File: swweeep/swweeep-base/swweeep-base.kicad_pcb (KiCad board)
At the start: 2 copper layers, 113.3 x 89.7 mm, 3 parts

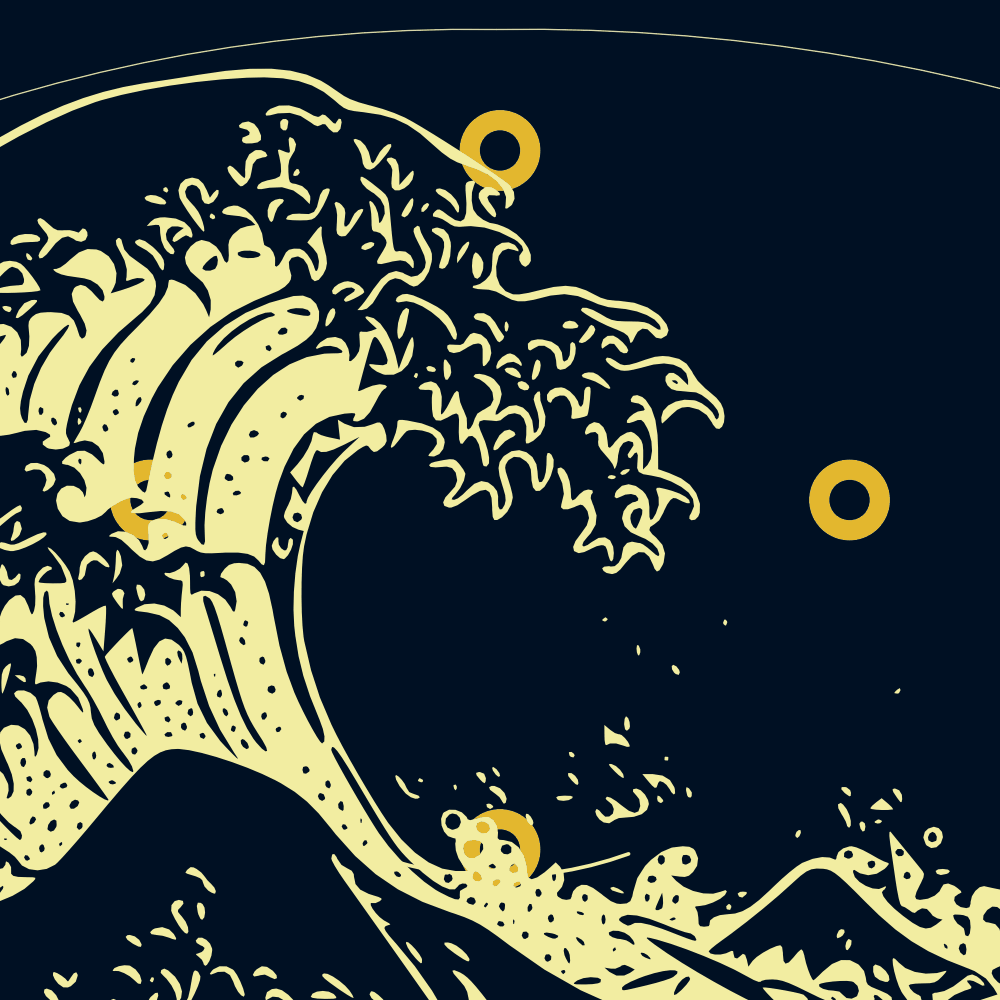
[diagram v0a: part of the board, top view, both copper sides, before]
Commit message: Mess up everything
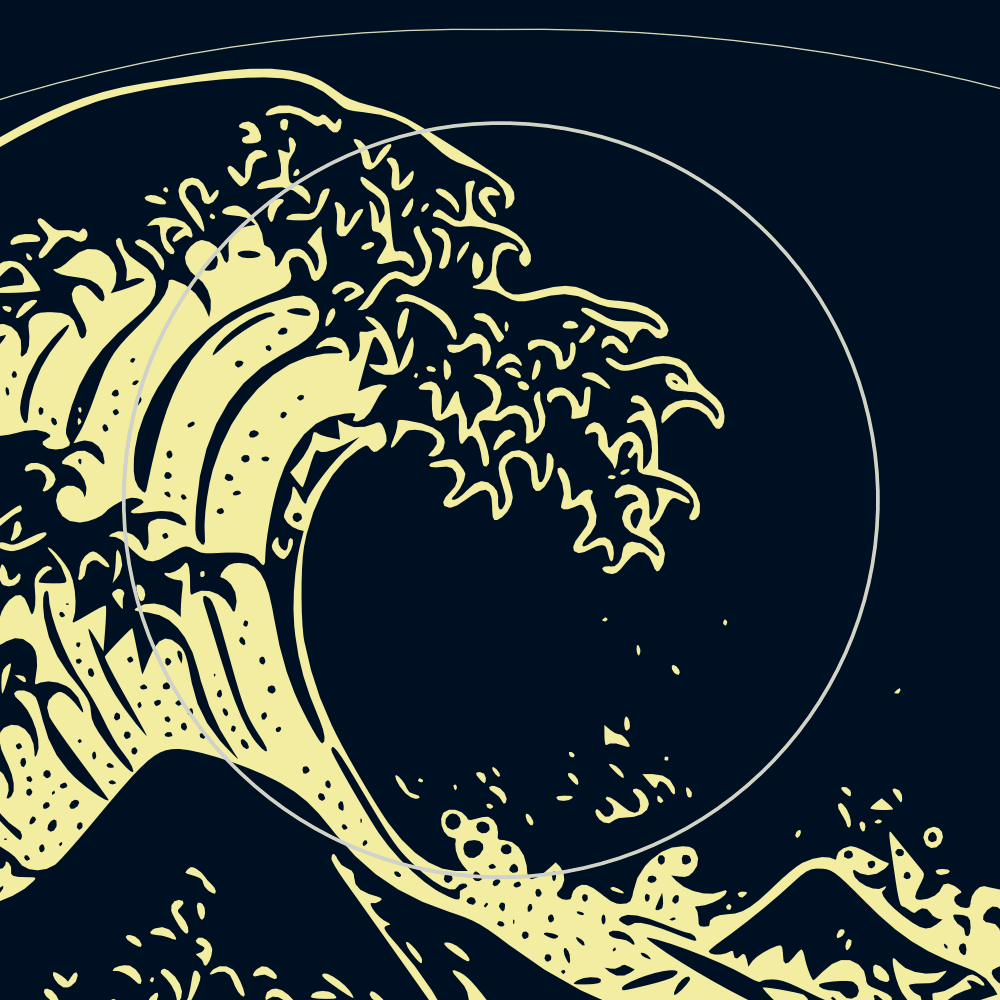
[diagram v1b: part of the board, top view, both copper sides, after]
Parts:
- removed REF**: Tenting Puck, kbd:Tenting_Puck2
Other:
- outline, holes or cut-outs redrawn
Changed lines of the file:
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@@
-(kicad_pcb (version 20230517) (generator pcbnew)
+(kicad_pcb (version 20230620) (generator pcbnew)
   (general
     (thickness 1.6)
@@
   (footprint "LOGO" (layer "F.Cu")
     (at 69.652089 50.051717)
-    (attr board_only exclude_from_pos_files exclude_from_bom)
-    (fp_text reference "G***1" (at 0 0 360) (layer "B.SilkS") hide
+    (property "Reference" "G***1" (at 0 0 0) (layer "B.SilkS") hide
       (effects (font (size 1.5 1.5) (thickness 0.3)) (justify mirror))
     )
-    (fp_text value "LOGO" (at 0.75 0 360) (layer "B.SilkS") hide
+    (property "Value" "LOGO" (at 0.75 0 0) (layer "B.SilkS") hide
       (effects (font (size 1.5 1.5) (thickness 0.3)) (justify mirror))
     )
+    (property "Footprint" "" (at 0 0 0 unlocked) (layer "F.Fab") hide
+      (effects (font (size 1 1) (thickness 0.15)))
+    )
+    (property "Datasheet" "" (at 0 0 0 unlocked) (layer "F.Fab") hide
+      (effects (font (size 1 1) (thickness 0.15)))
+    )
+    (property "Description" "" (at 0 0 0 unlocked) (layer "F.Fab") hide
+      (effects (font (size 1.5 1.5) (thickness 0.3)))
+    )
+    (attr board_only exclude_from_pos_files exclude_from_bom)
     (fp_poly
       (pts
@@
       (stroke (width 0) (type solid)) (fill solid) (layer "F.SilkS"))
   )
-  (footprint "kbd:Tenting_Puck2" (layer "F.Cu")
-    (at 68.280606 38.5986)
-    (attr through_hole)
-    (fp_text reference "REF**" (at 7.6835 1.4605) (layer "F.Fab")
-      (effects (font (size 1 1) (thickness 0.15)))
-    )
-    (fp_text value "Tenting Puck" (at 8.0645 -2.8575) (layer "F.Fab")
-      (effects (font (size 1 1) (thickness 0.15)))
-    )
-    (fp_arc (start -2.8575 20.32) (mid -4.959785 19.91151) (end -7.008045 19.286135)
-      (stroke (width 0.2) (type solid)) (layer "B.SilkS"))
-    (fp_arc (start 7.008045 19.286135) (mid 4.959785 19.91151) (end 2.8575 20.32)
-      (stroke (width 0.2) (type solid)) (layer "B.SilkS"))
-    (fp_arc (start -2.8575 20.32) (mid -4.959785 19.91151) (end -7.008046 19.286135)
-      (stroke (width 0.2) (type solid)) (layer "F.SilkS"))
-    (fp_arc (start 7.008047 19.286134) (mid 4.959786 19.91151) (end 2.8575 20.32)
-      (stroke (width 0.2) (type solid)) (layer "F.SilkS"))
-    (fp_line (start -17.6 10) (end -17.6 -10)
-      (stroke (width 0.2) (type solid)) (layer "Cmts.User"))
-    (fp_line (start -1.6 19.05) (end -1.6 -19.05)
-      (stroke (width 0.2) (type solid)) (layer "Cmts.User"))
-    (fp_line (start 1.6 19.05) (end 1.6 -19.05)
-      (stroke (width 0.2) (type solid)) (layer "Cmts.User"))
-    (fp_line (start 17.6 10) (end 17.6 -10)
-      (stroke (width 0.2) (type solid)) (layer "Cmts.User"))
-    (fp_circle (center 0 0) (end 20.55 0)
-      (stroke (width 0.55) (type solid)) (fill none) (layer "B.CrtYd"))
-    (fp_text user " " (at -0.254 -6.9215 90) (layer "B.SilkS") hide
-      (effects (font (size 1 1) (thickness 0.1)) (justify mirror))
-    )
-    (fp_text user "  " (at -0.254 -6.0325 90) (layer "F.SilkS") hide
-      (effects (font (size 1 1) (thickness 0.1)))
-    )
-    (pad "1" thru_hole circle (at -19.05 0) (size 4.4 4.4) (drill 2.2) (layers "*.Cu" "*.Mask"))
-    (pad "1" thru_hole circle (at 0 -19.05) (size 4.4 4.4) (drill 2.2) (layers "*.Cu" "*.Mask"))
-    (pad "1" thru_hole circle (at 0 19.05) (size 4.4 4.4) (drill 2.2) (layers "*.Cu" "*.Mask"))
-    (pad "1" thru_hole circle (at 19.05 0) (size 4.4 4.4) (drill 2.2) (layers "*.Cu" "*.Mask"))
-  )
   (footprint "LOGO" (layer "B.Cu")
     (at 69.596 50.038 180)
-    (attr board_only exclude_from_pos_files exclude_from_bom)
-    (fp_text reference "G***" (at 0 0 180) (layer "B.SilkS") hide
+    (property "Reference" "G***" (at 0 0 180) (layer "B.SilkS") hide
       (effects (font (size 1.5 1.5) (thickness 0.3)) (justify mirror))
     )
-    (fp_text value "LOGO" (at -0.75 0 180) (layer "B.SilkS") hide
+    (property "Value" "LOGO" (at -0.75 0 180) (layer "B.SilkS") hide
       (effects (font (size 1.5 1.5) (thickness 0.3)) (justify mirror))
     )
+    (property "Footprint" "" (at 0 0 180 unlocked) (layer "F.Fab") hide
+      (effects (font (size 1 1) (thickness 0.15)))
+    )
+    (property "Datasheet" "" (at 0 0 180 unlocked) (layer "F.Fab") hide
+      (effects (font (size 1 1) (thickness 0.15)))
+    )
+    (property "Description" "" (at 0 0 180 unlocked) (layer "F.Fab") hide
+      (effects (font (size 1.5 1.5) (thickness 0.3)))
+    )
+    (attr board_only exclude_from_pos_files exclude_from_bom)
     (fp_poly
       (pts
@@
   (gr_arc (start 13.8176 30.5816) (mid 39.482162 17.252631) (end 68.080607 12.956108)
     (stroke (width 0.05) (type solid)) (layer "Edge.Cuts"))
+  (gr_circle (center 68.326 38.608) (end 88.876 38.608)
+    (stroke (width 0.2) (type solid)) (fill solid) (layer "Edge.Cuts"))
   (gr_arc (start 14.468605 83.699722) (mid 13.081165 83.190716) (end 12.430857 81.863623)
     (stroke (width 0.05) (type solid)) (layer "Edge.Cuts"))
